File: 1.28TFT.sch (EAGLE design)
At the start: 15 parts, among them M1 LCD_FPCST, X1 1X7FFC

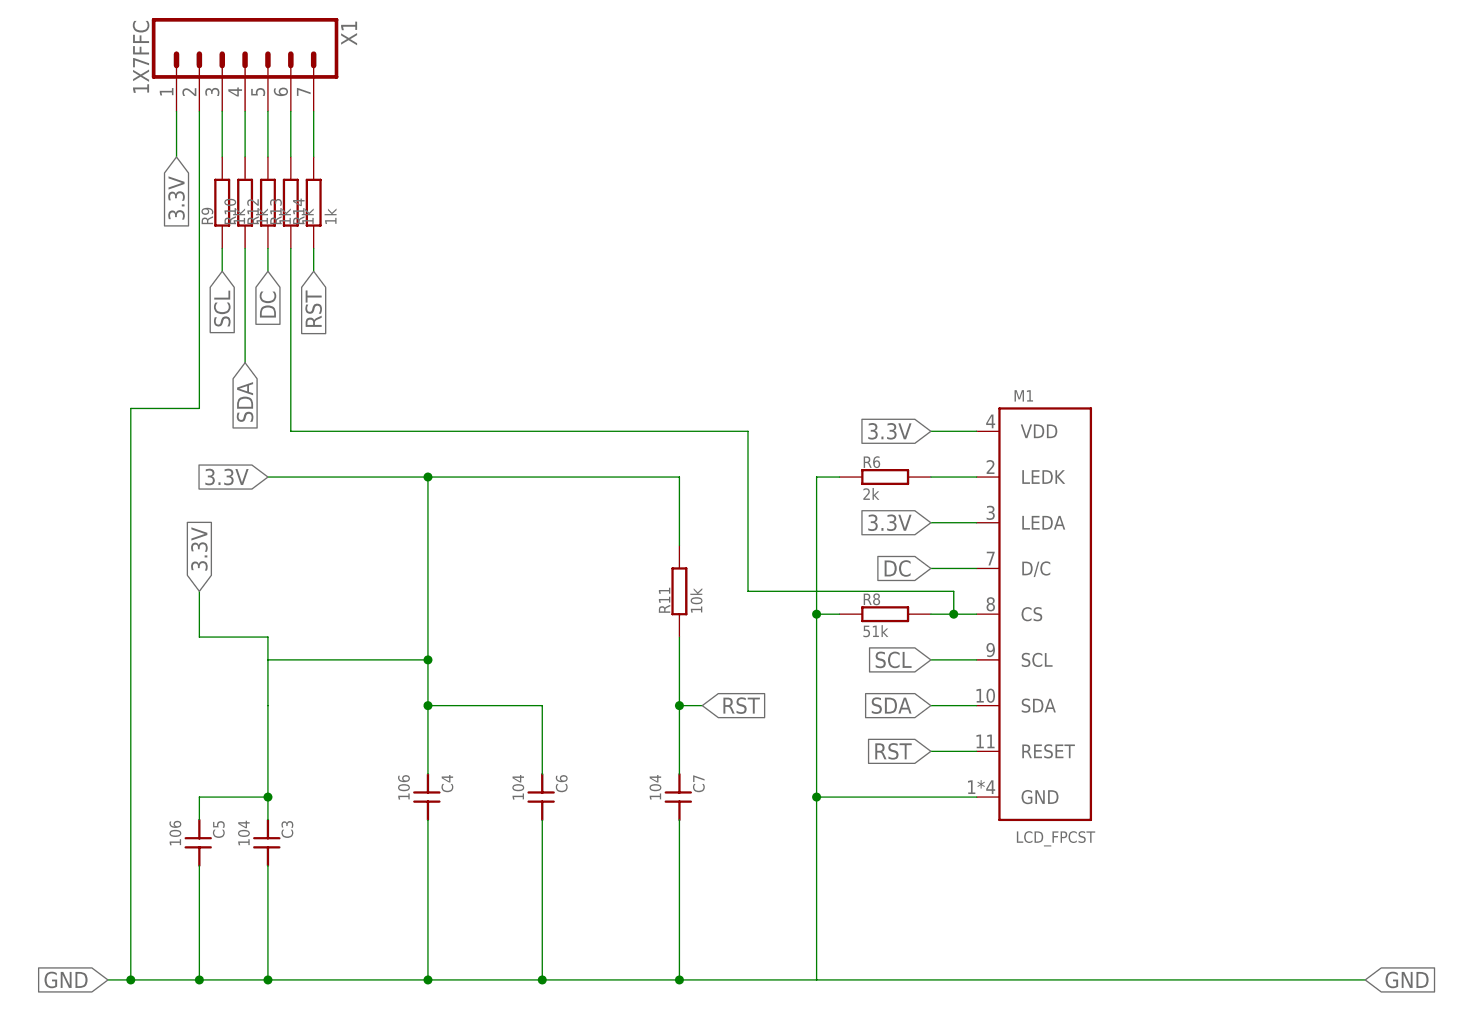
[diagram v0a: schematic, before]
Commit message: BUGFIX
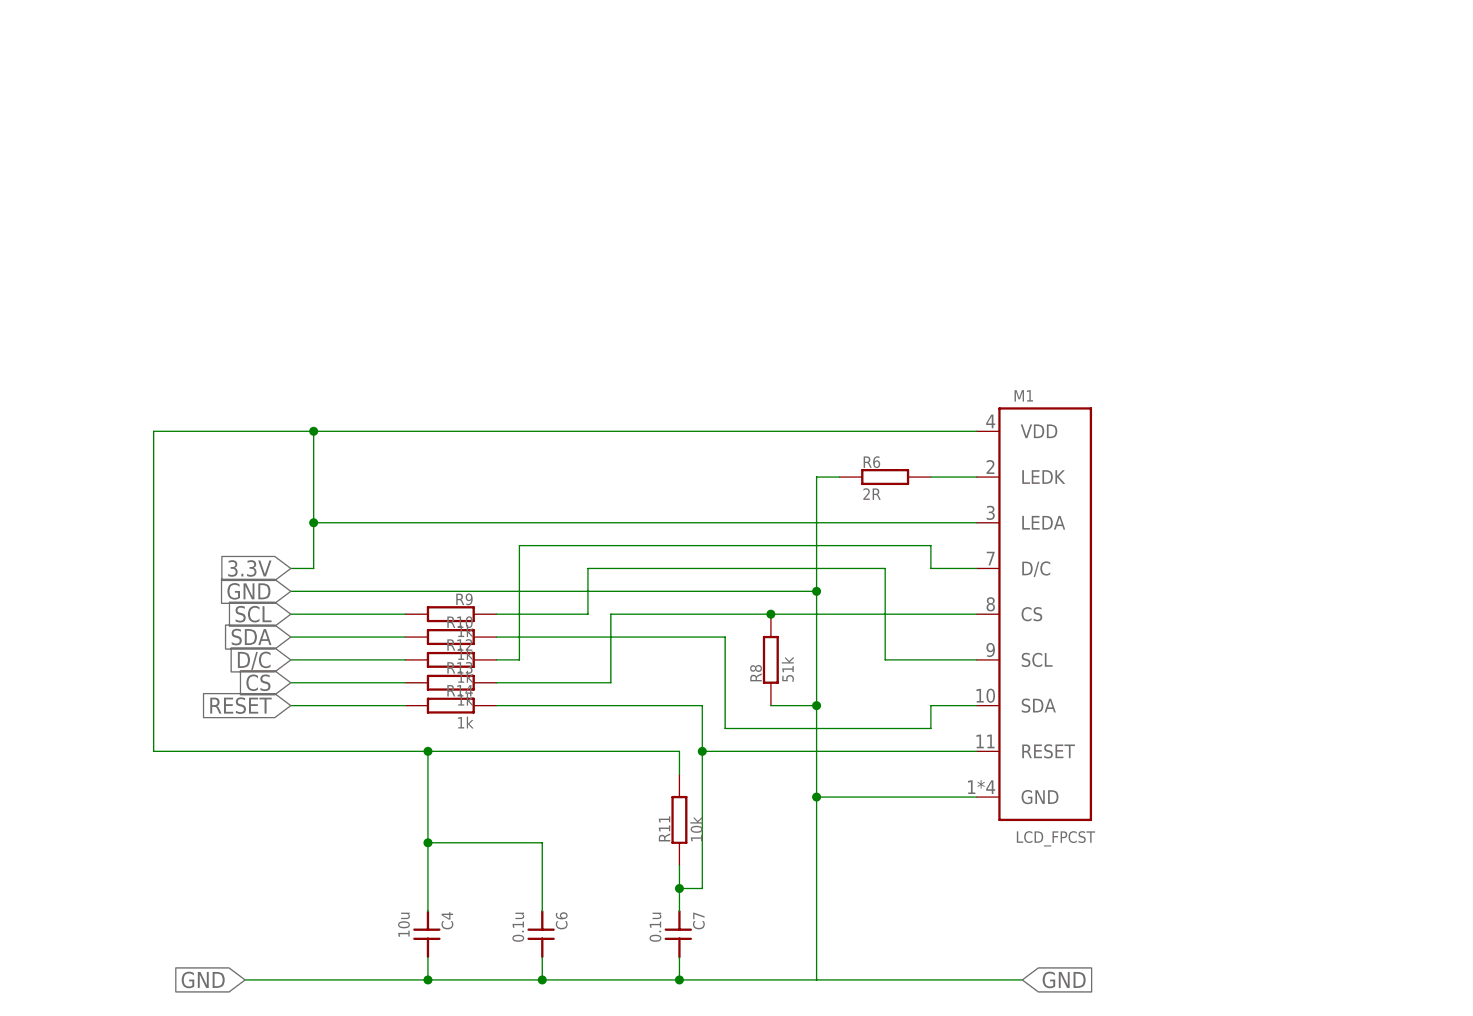
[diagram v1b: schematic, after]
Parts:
- removed C3: 104, LARS_409_R,C,L:C0603
- removed C5: 106, LARS_409_R,C,L:C0603
- removed X1: 1X7FFC, LARS_409_CONNECTORS:1X7FFC
- C4: value 106 -> 10u
- C6, C7: value 104 -> 0.1u
- R6: value 2k -> 2R
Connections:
- removed net N$3: R9.P$2, X1.3
- removed net N$4: R10.P$2, X1.4
- removed net N$6: R12.P$2, X1.5
- removed net N$7: R13.P$2, X1.6
- removed net N$8: R14.P$2, X1.7
- new net CS: R13.P$2
- new net D/C: R12.P$2
- new net RESET: R14.P$2
- net 3.3V: no longer C3.P$1, C5.P$1, X1.1
- net GND: no longer C3.P$2, C5.P$2, X1.2
- net SCL: now also R9.P$2
- net SDA: now also R10.P$2
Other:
- moved on the sheet: C4, C6, C7, R10, R11, R12, R13, R14, R8, R9
